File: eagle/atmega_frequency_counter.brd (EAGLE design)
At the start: 100 x 80 mm, 49 parts, among them IC1 TL071P, IC2 TL072P, T1 2N3904, U1 ATMEGA328P_PDIP

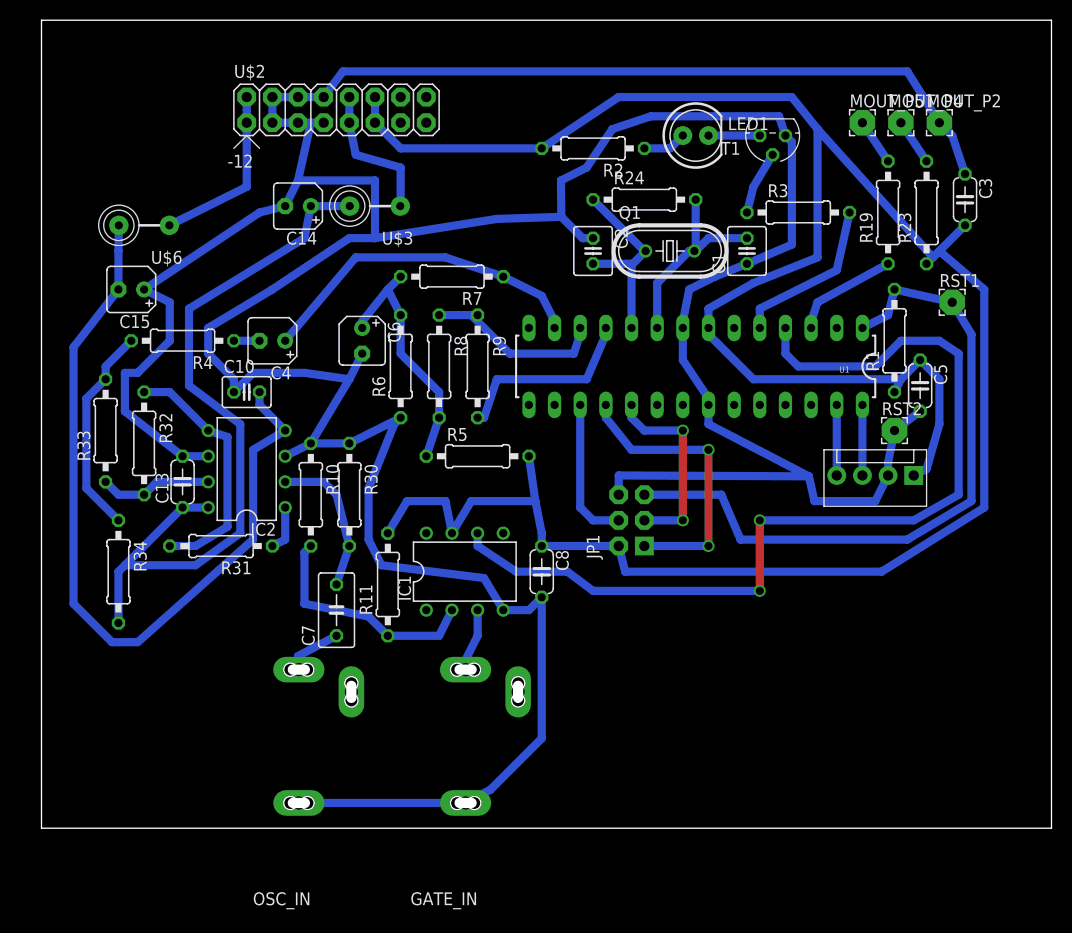
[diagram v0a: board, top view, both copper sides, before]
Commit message: layout
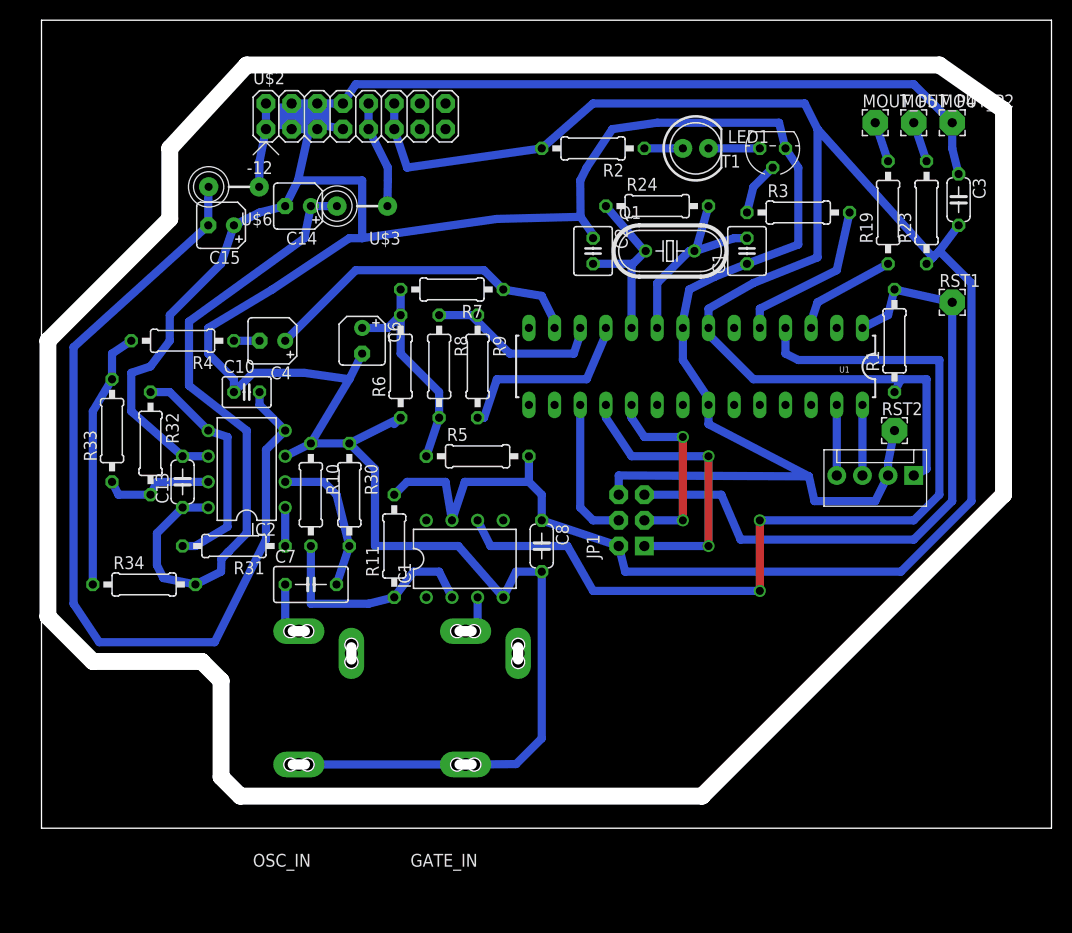
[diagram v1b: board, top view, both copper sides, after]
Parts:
- removed C5: .1uF, rcl:C050-024X044
- moved C15 10.9 mm to (17.8, 59.7)
- moved U$6 9.67 mm to (19.1, 63.5)
- moved R11 3.86 mm to (34.9, 27.9)
- moved GATE_IN 3.81 mm to (47.0, 3.81)
- moved OSC_IN 3.81 mm to (30.5, 3.81)
- moved C7 3.59 mm to (26.7, 24.1), turned to 0 degrees
- moved R34 2.84 mm to (10.2, 24.1), turned to 0 degrees
- moved C8 2.54 mm to (49.5, 27.9)
- moved U$2 2.01 mm to (28.6, 70.5)
- moved R24 1.42 mm to (61.0, 61.6)
- moved IC1 1.27 mm to (41.9, 26.7)
- moved U$3 1.27 mm to (31.8, 61.6)
- moved R31 1.27 mm to (19.1, 27.9)
- moved LED1 1.27 mm to (64.8, 67.3)
- moved MOUT_P2 1.27 mm to (90.2, 69.8)
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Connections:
- net +5V: no longer C5.1
- net GND: no longer C5.2
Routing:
- net GND: track 423.5 -> 411.7 mm
- net -12V: track 79.7 -> 91.0 mm
- net N$37: track 17.4 -> 8.32 mm
- net +12V: track 74.3 -> 65.5 mm
- net +5V: track 243.2 -> 235.6 mm
- net N$62: track 20.9 -> 25.7 mm
- net N$17: track 93.6 -> 89.2 mm
- net N$34: track 14.3 -> 10.6 mm
- net N$12: track 25.1 -> 22.6 mm
- net N$43: track 67.9 -> 66.0 mm
- net N$60: track 25.1 -> 23.2 mm
- net N$5: track 19.4 -> 18.1 mm
- net N$6: track 6.32 -> 5.31 mm
- net N$11: track 33.5 -> 32.6 mm
- net N$59: track 4.59 -> 3.81 mm
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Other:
- outline, holes or cut-outs redrawn

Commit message: layout
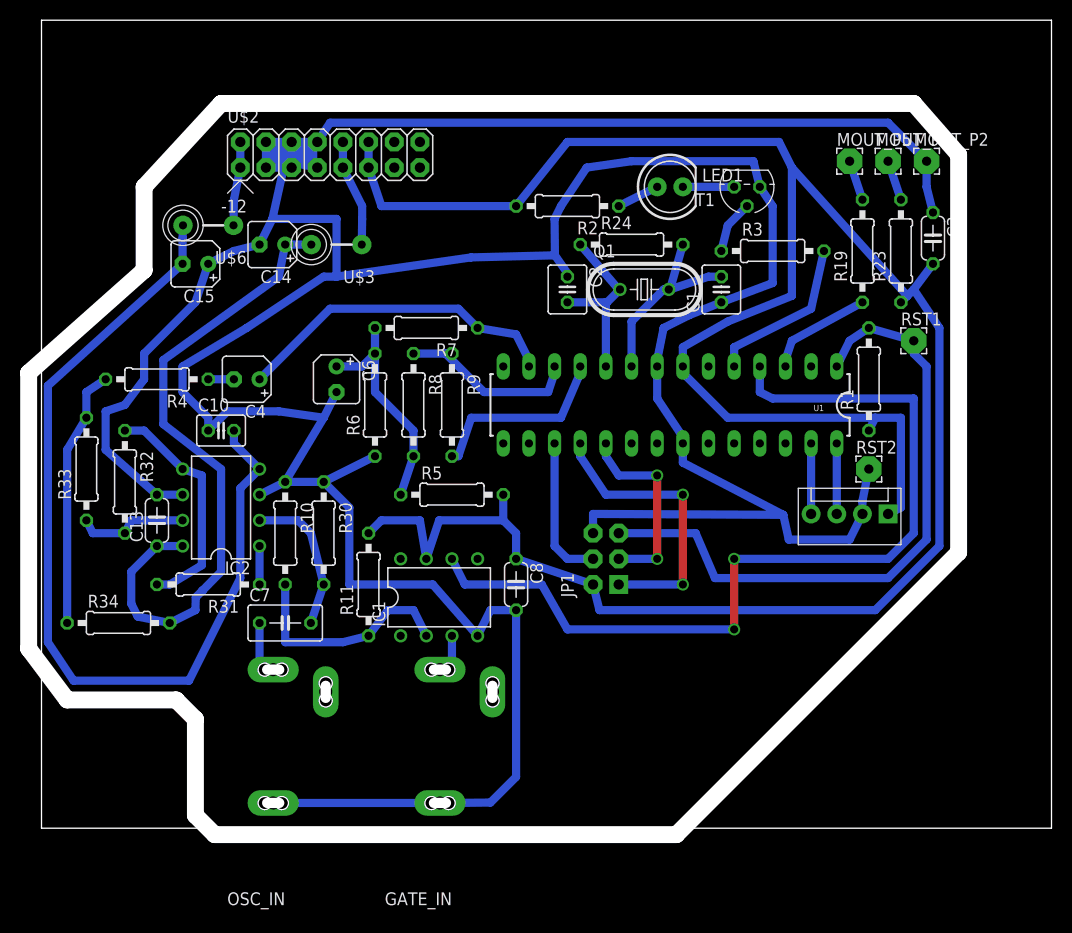
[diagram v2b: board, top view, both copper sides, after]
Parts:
- moved R2 6.25 mm to (52.1, 61.6)
- moved RST1 5.39 mm to (86.4, 48.3)
- moved R3 4.58 mm to (72.4, 57.1)
- moved T1 4.58 mm to (69.8, 63.5)
- moved R10 4.58 mm to (24.1, 29.2)
- moved C10 4.58 mm to (17.8, 39.4)
- moved C14 4.58 mm to (22.9, 57.8)
- moved C8 4.58 mm to (47.0, 24.1)
- moved IC1 4.58 mm to (39.4, 22.9)
- moved IC2 4.58 mm to (17.8, 31.8)
- moved LED1 4.58 mm to (62.2, 63.5)
- moved R11 4.58 mm to (32.4, 24.1)
- moved R24 4.58 mm to (58.4, 57.8)
- moved R30 4.58 mm to (27.9, 29.2)
- moved R31 4.58 mm to (16.5, 24.1)
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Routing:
- net N$43: track 66.0 -> 65.0 mm
- net GND: track 411.7 -> 410.8 mm
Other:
- board size 100 x 80 mm -> 101.3 x 80.6 mm

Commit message: tweaked
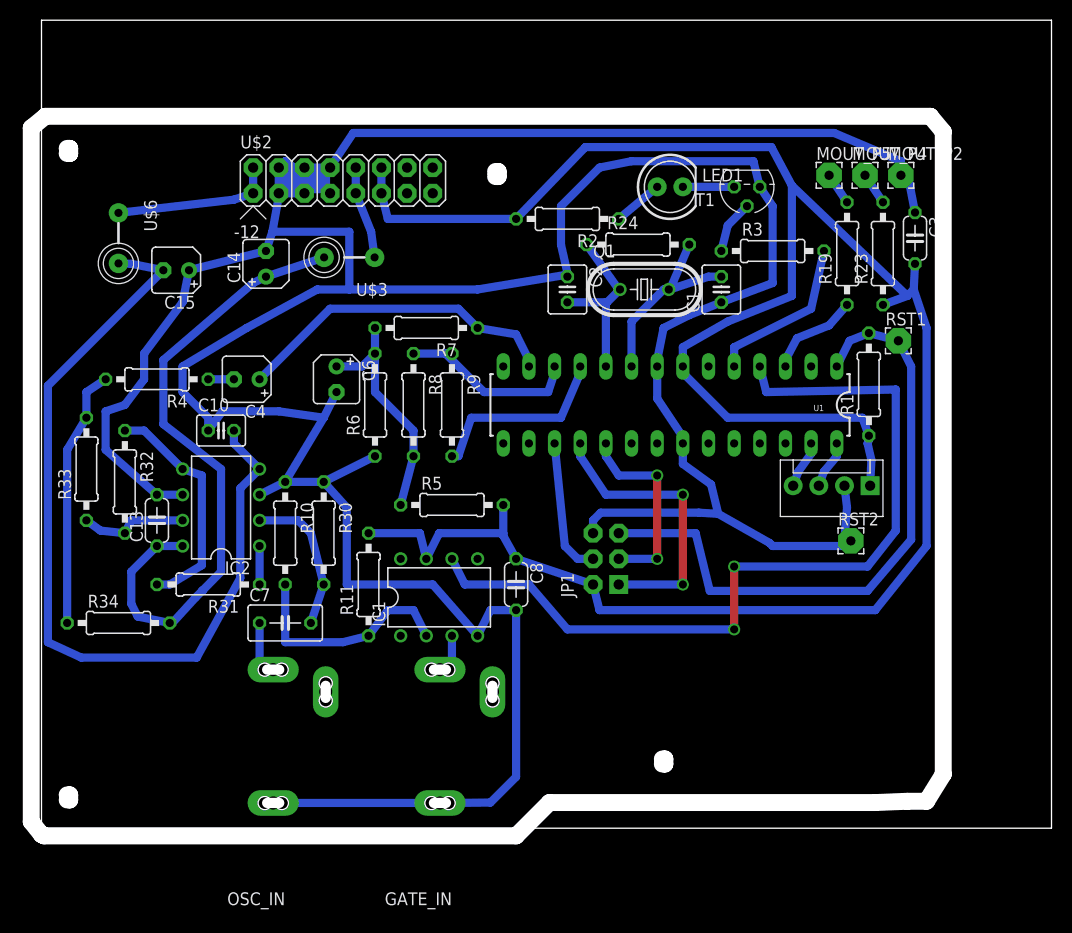
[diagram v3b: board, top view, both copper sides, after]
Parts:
- moved U$6 8.98 mm to (7.62, 58.4), turned to 270 degrees
- moved RST2 7.33 mm to (80.1, 28.4)
- moved DISPLAY 3.31 mm to (82.0, 33.9)
- moved MOUT_P2 2.90 mm to (85.1, 64.6)
- moved U$2 2.84 mm to (27.3, 64.1)
- moved MOUT_P4 2.68 mm to (81.5, 64.6)
- moved MOUT_P5 2.47 mm to (78.0, 64.6)
- moved C15 2.01 mm to (13.3, 55.2)
- moved C14 2.01 mm to (22.2, 55.9), turned to 90 degrees
- moved R23 1.80 mm to (83.3, 56.9)
- moved U$3 1.80 mm to (30.5, 56.5)
- moved C3 1.78 mm to (86.5, 58.4)
- moved R19 1.55 mm to (79.8, 56.9)
- moved RST1 1.52 mm to (84.8, 48.3)
- moved R2 1.27 mm to (52.1, 60.3)
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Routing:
- net +5V: track 236.1 -> 218.6 mm
- net N$37: track 8.32 -> 16.1 mm
- net -12V: track 91.0 -> 86.6 mm
- net N$17: track 89.2 -> 84.9 mm
- net GND: track 410.8 -> 407.7 mm
- net N$3: track 6.99 -> 4.69 mm
- net N$2: track 6.99 -> 4.74 mm
- net N$34: track 10.6 -> 9.21 mm
- net N$57: track 10.6 -> 9.20 mm
- net N$43: track 65.0 -> 63.7 mm
- net +12V: track 65.5 -> 64.3 mm
- net N$12: track 22.6 -> 23.6 mm
- net N$26: track 14.5 -> 13.5 mm
- net N$55: track 4.02 -> 3.21 mm
- net N$46: track 4.02 -> 3.21 mm
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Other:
- board size 101.3 x 80.6 mm -> 101 x 80.8 mm
